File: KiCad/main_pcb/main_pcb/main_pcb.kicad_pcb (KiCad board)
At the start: 2 copper layers, 92.3 x 80.5 mm, 49 parts, among them J1 Conn_01x06, J2 Conn_01x21, J3 Conn_01x13, J4 Conn_01x07, J5 Conn_01x07, J6 USB_C_Receptacle_USB2.0_14P, J7 Conn_01x01, J8 Conn_01x01, SW1 SW_Push, U1 ATmega2560-16A, U2 TXB0104D, U3 TXB0104D, U4 TXB0104D, U5 CH340C, U6 AMS1117-3.3, Y1 Crystal_GND24

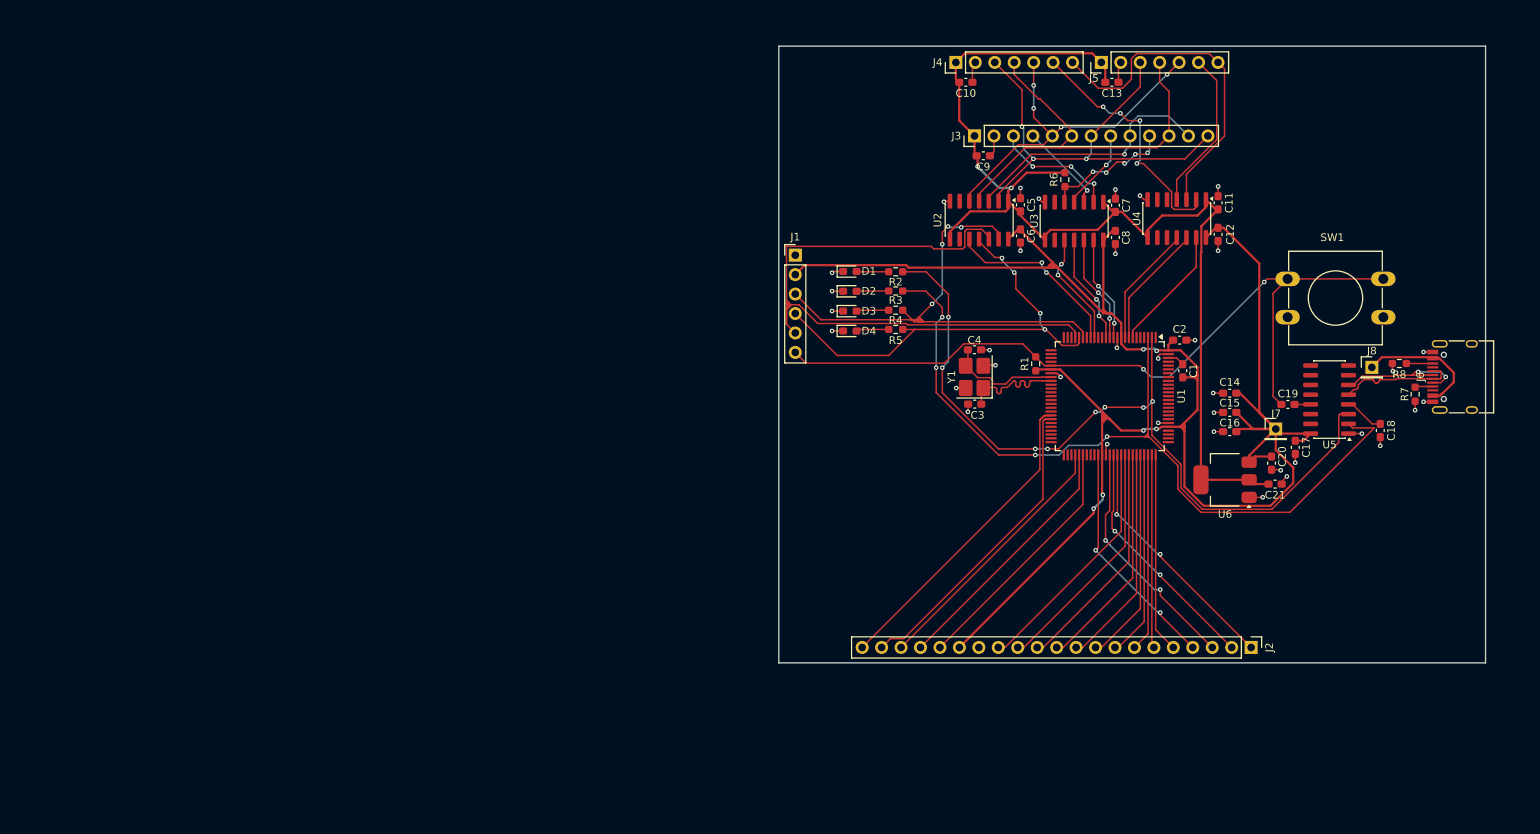
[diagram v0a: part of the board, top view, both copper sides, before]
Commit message: feat(pcb): Second draft
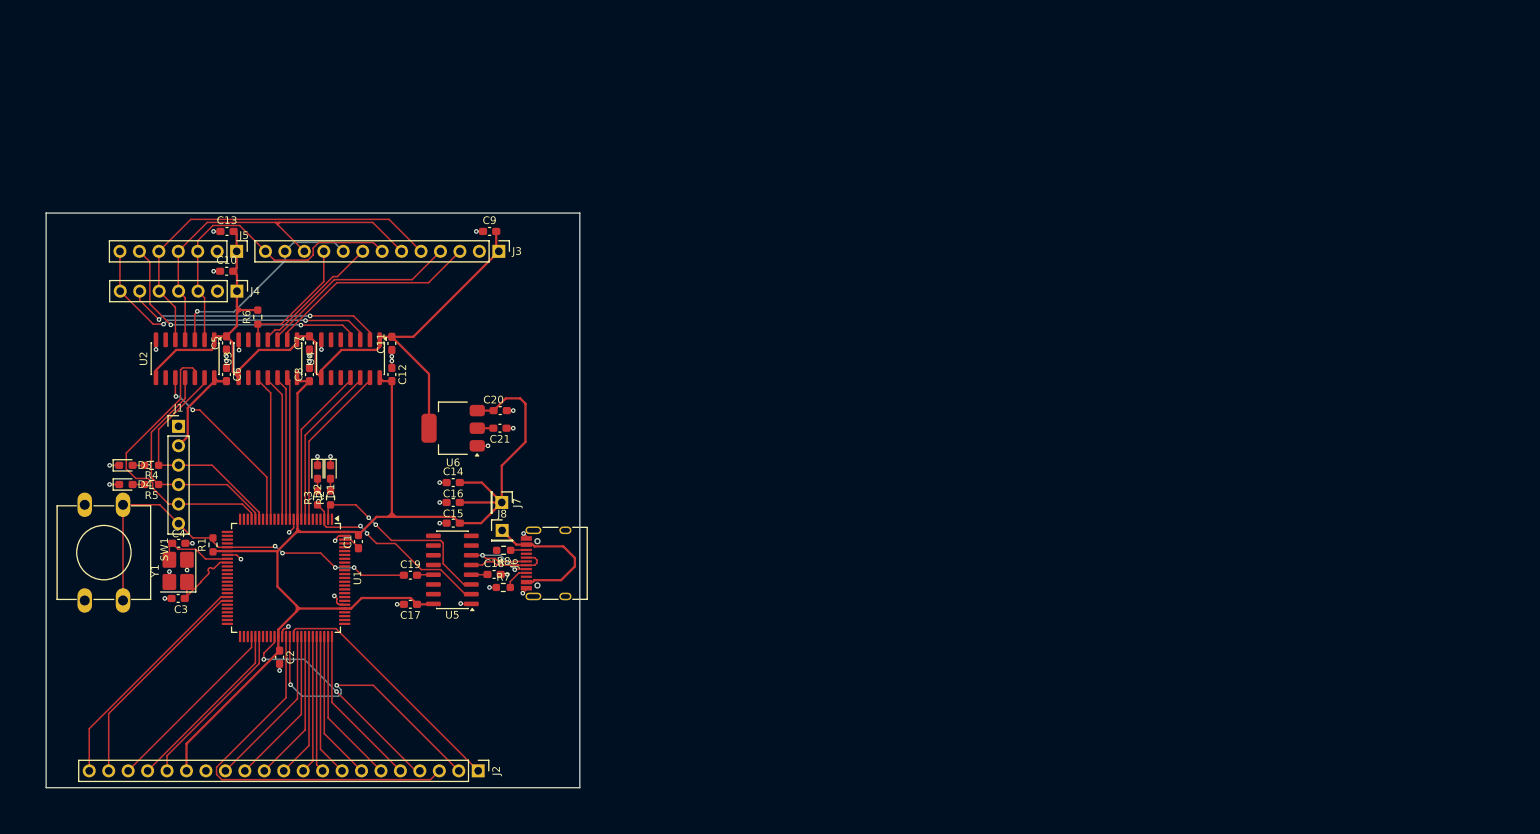
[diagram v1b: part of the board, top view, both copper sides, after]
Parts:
- moved SW1 154.9 mm to (68.4, 99.7), turned to -90 degrees
- moved C2 124.6 mm to (88.8, 119.6), turned to -90 degrees
- moved R7 121.7 mm to (118.1, 110.5), turned to 180 degrees
- moved J6 120.9 mm to (125.1, 107.3)
- moved R8 119.5 mm to (118.1, 105.7)
- moved C17 117.4 mm to (105.9, 112.7), turned to 180 degrees
- moved C18 117.3 mm to (116.9, 108.8), turned to 0 degrees
- moved C13 117.2 mm to (82.0, 64.0), turned to 0 degrees
- moved C19 116.7 mm to (105.9, 108.9)
- moved U5 116.7 mm to (111.4, 108.2)
- moved J5 115.6 mm to (83.2, 66.6), turned to -90 degrees
- moved J8 115.6 mm to (117.9, 103.0)
- moved U1 110.2 mm to (89.7, 109.2)
- moved R1 110.0 mm to (80.2, 104.9)
- moved C1 109.9 mm to (99.2, 104.5), turned to -90 degrees
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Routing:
- net /USB-C/TXD: track 107.3 -> 26.2 mm, vias 4 -> 2
- net /USB-C/RXD: track 105.0 -> 26.3 mm, vias 8 -> 2
- net VCC: track 262.4 -> 187.7 mm, vias 6 -> 0
- net /USB-C/USB-C_RST: track 103.1 -> 53.4 mm, vias 2 -> 4
- net /MISO: track 87.6 -> 38.9 mm
- net 3V3: track 144.3 -> 105.7 mm, vias 2 -> 0
- net /SCK: track 68.7 -> 30.5 mm, vias 4 -> 0
- net /MOSI: track 59.6 -> 31.2 mm, vias 4 -> 0
- net /R3: track 31.6 -> 51.6 mm, vias 2 -> 0
- net /Screens/SCK_3V3: track 61.7 -> 42.0 mm, vias 3 -> 0
- net Net-(J5-Pin_6): track 21.1 -> 36.1 mm, vias 0 -> 2
- net Net-(J3-Pin_4): track 11.8 -> 26.3 mm, vias 1 -> 0
- net /SDA: track 41.6 -> 29.1 mm
- net /SCL: track 42.7 -> 30.7 mm
- net Net-(J3-Pin_3): track 16.4 -> 27.9 mm, vias 3 -> 0
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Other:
- board size 92.3 x 80.5 mm -> 69.7 x 75.1 mm
